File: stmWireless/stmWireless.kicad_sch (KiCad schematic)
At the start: 36 parts, among them IC1 BALFLB-WL-08D3, J1 SWD, J2 CORTEX_DEBUG, J3 Conn_02x08_Top_Bottom, U1 STM32WLE5CBU6, U2 AP63203WU, Y1 Crystal_32MHz, Y2 Crystal_32.768kHz

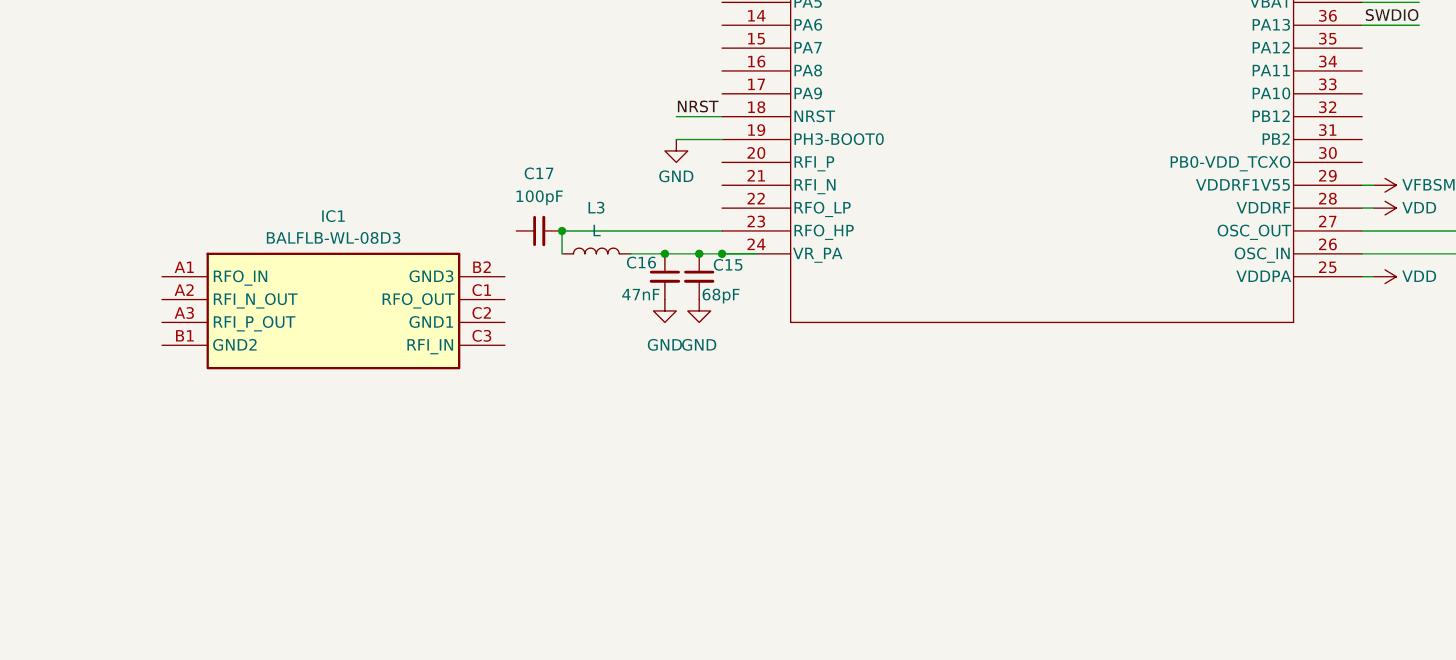
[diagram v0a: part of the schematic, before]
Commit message: more wiorless
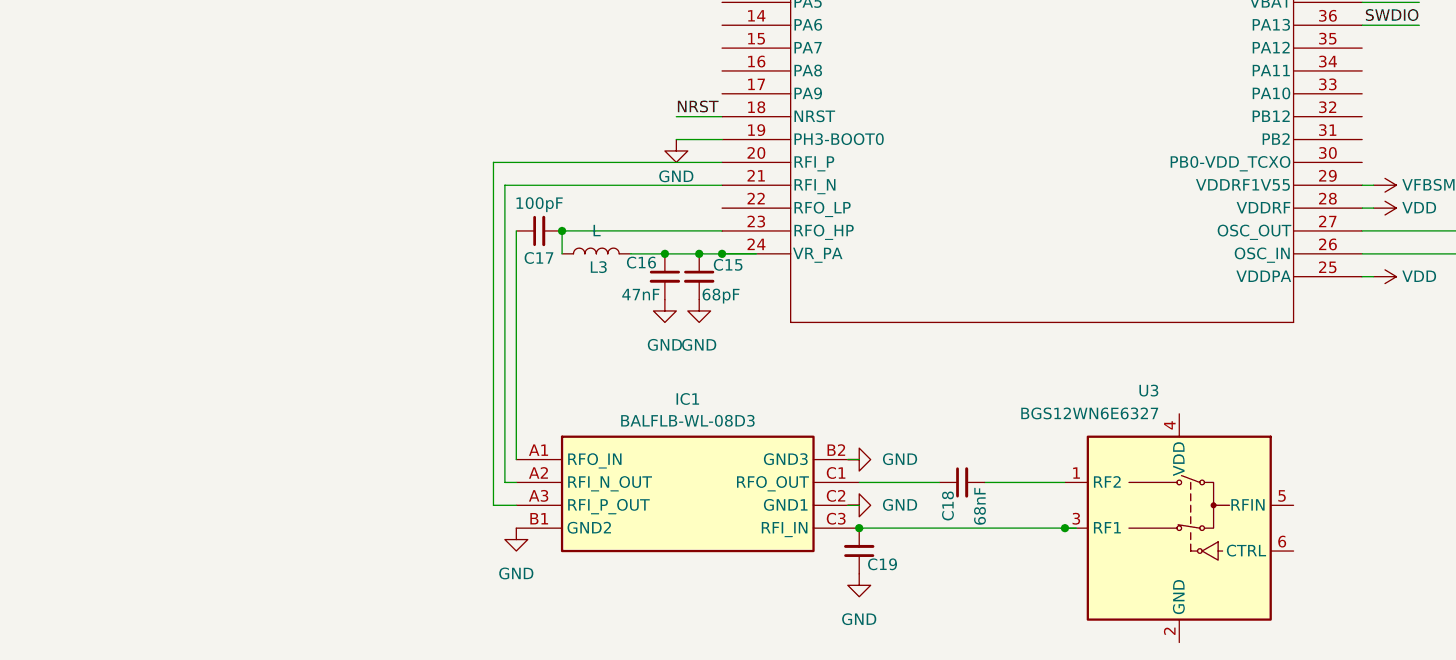
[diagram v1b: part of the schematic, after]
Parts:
- added C18: 68nF, symbol Device:C_Small
- added C19: ~, symbol Device:C_Small
- added U3: BGS12WN6E6327, Package_LGA:Infineon_PG-TSNP-6-10_0.7x1.1mm_0.7x1.1mm_P0.4mm, symbol RF_Switch:BGS12WN6E6327
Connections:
- net GND: now also IC1.B1 (GND2), IC1.B2 (GND3), IC1.C2 (GND1), C19.1
- net at IC1.A1 (RFO_IN): now also C17.1
- net at IC1.A2 (RFI_N_OUT): now also U1.21 (RFI_N)
- net at IC1.A3 (RFI_P_OUT): now also U1.20 (RFI_P)
- net at IC1.C1 (RFO_OUT): now also C18.1
- net at IC1.C3 (RFI_IN): now also C19.2, U3.3 (RF1)
- new net: C18.2, U3.1 (RF2)
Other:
- moved on the sheet: IC1
